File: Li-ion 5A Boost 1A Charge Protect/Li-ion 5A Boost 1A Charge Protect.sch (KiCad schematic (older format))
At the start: 44 parts, among them J1 USB_C_FEMALE, SW1 SW_SPST, U1 AP9101CK6, U2 ECH8695R-TL-W, U3 MCP73833T, U4 PAM2423AECADJR

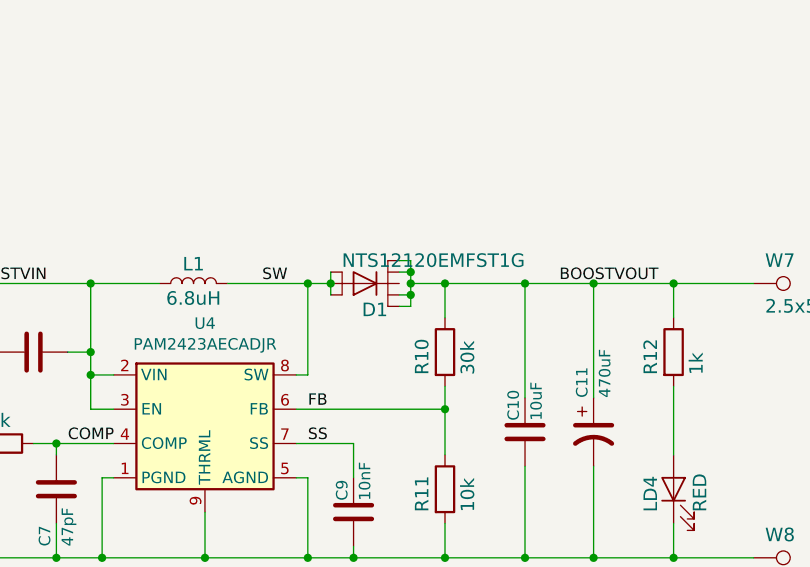
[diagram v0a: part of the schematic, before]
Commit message: PCB Before Solder Footprint Switch
Before switching wire solder points to foot prints with through holes.
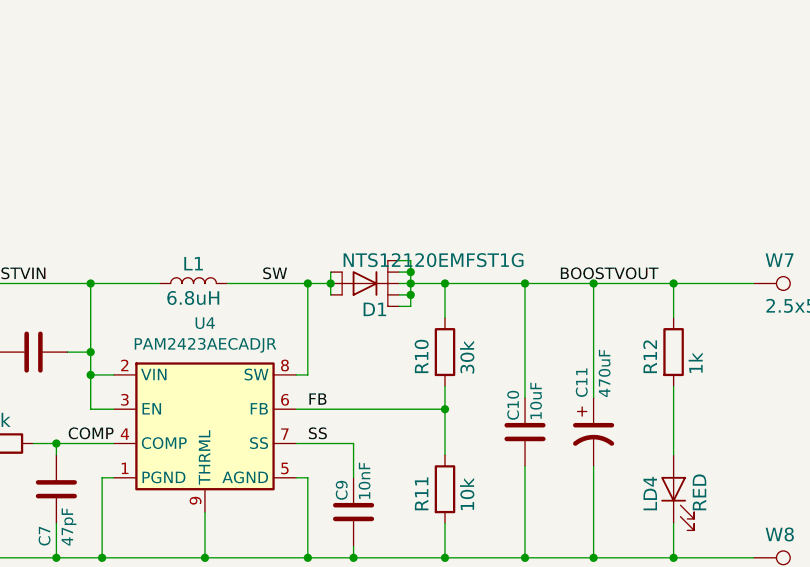
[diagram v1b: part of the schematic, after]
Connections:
- wire segments 177 -> 178
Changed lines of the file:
@@
 Wire Wire Line
 	10050 5000 10050 5050
-Connection ~ 10550 5000
 Wire Wire Line
 	10350 5050 10400 5050
-Wire Wire Line
-	10350 4950 10400 4950
-Wire Wire Line
-	10350 4900 10400 4900
-Wire Wire Line
-	10400 4950 10400 5000
 Wire Wire Line
 	10350 5100 10400 5100
 Wire Wire Line
 	10400 5050 10400 5000
-Connection ~ 10400 5000
-Wire Wire Line
-	10400 5000 10550 5000
 Wire Wire Line
 	10400 5050 10400 5100
 Connection ~ 10400 5050
+Text Label 4000 5150 0    50   ~ 0
+PVM
+Wire Wire Line
+	10400 5000 10350 5000
+Connection ~ 10400 5000
+Connection ~ 10550 5000
+Wire Wire Line
+	10400 5000 10550 5000
+Connection ~ 10400 4950
+Wire Wire Line
+	10400 4950 10400 5000
+Wire Wire Line
+	10350 4950 10400 4950
 Wire Wire Line
 	10400 4950 10400 4900
-Connection ~ 10400 4950
-Text Label 4000 5150 0    50   ~ 0
-PVM
+Wire Wire Line
+	10350 4900 10400 4900
 $EndSCHEMATC
